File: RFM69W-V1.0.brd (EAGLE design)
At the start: 19.2 x 30.8 mm, 14 parts, among them J1 NRF connector, J2 SD card

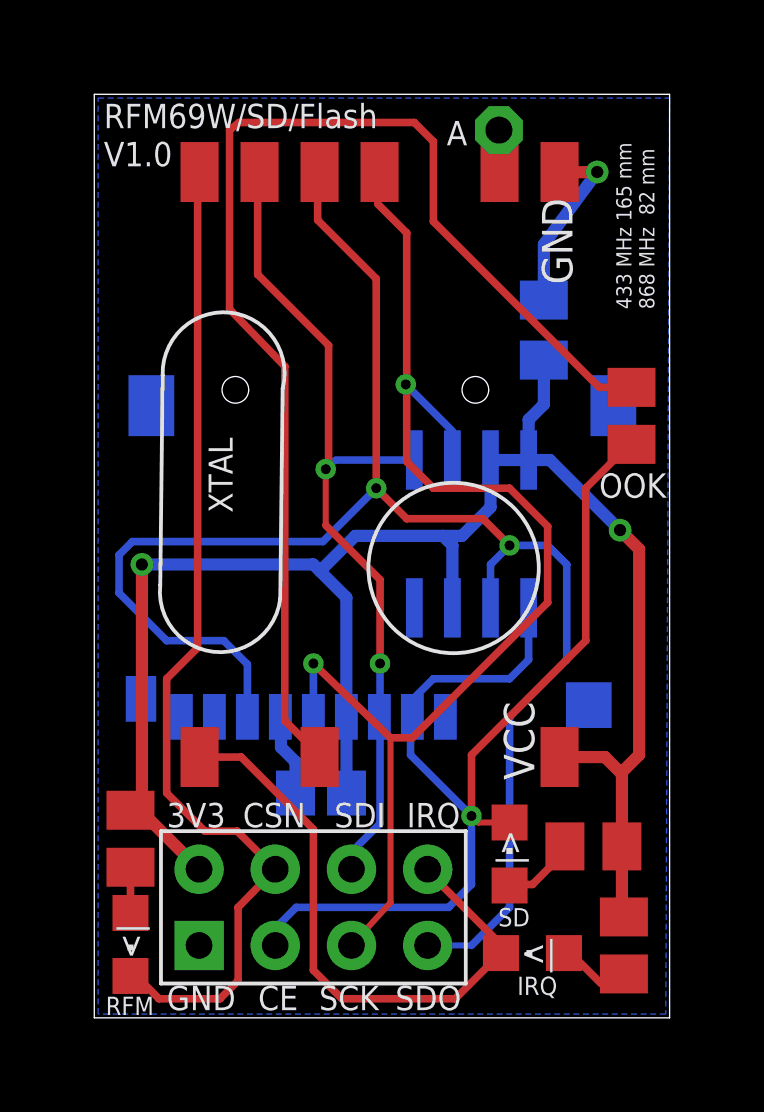
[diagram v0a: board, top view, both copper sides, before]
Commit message: Cosmetic update
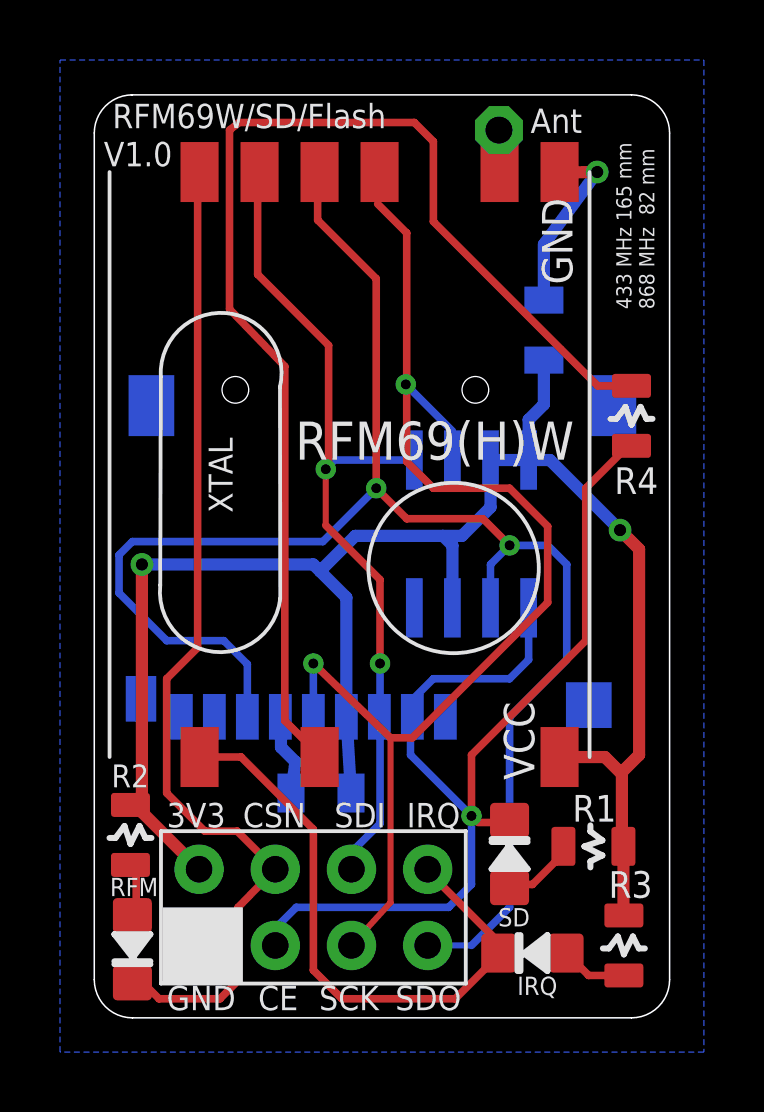
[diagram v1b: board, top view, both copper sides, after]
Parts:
- removed LED1: RED, dp_devices:LED-805
- removed LED2: GREEN, dp_devices:LED-805
- removed LED3: YELLOW, dp_devices:LED-805
- added U$2, U$3, U$4: LED0805-LARGE, _c2h:0805-LED-LARGEPADS
- C1: device resistor:C0805K -> _c2h:0805-CAP
- C2: device resistor:C0805 -> _c2h:0805-CAP
- R1, R2, R3, R4: device resistor:M0805 -> _c2h:0805-RES
- moved R2 0.13 mm to (1.33, 6.22)
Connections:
- net CE: now also U$2.MINUS; no longer LED1.C
- net CSN: now also U$3.MINUS; no longer LED2.C
- net IRQ: now also U$4.MINUS; no longer LED3.C
- net N$2: now also U$2.PLUS; no longer LED1.A
- net N$3: now also U$3.PLUS; no longer LED2.A
- net N$5: now also U$4.PLUS; no longer LED3.A
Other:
- outline, holes or cut-outs redrawn
- board text added: "Ant"
- board text added: "R1"
- board text added: "R2"
- board text added: "R3"
- board text added: "R4"
- board text added: "RFM69(H)W"
- board text removed: "<|"
- board text removed: "A"
- board text removed: "OOK"
- board text removed: "|>"
